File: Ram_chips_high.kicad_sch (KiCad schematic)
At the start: 10 parts, among them U25 MM5280, U26 MM5280, U27 MM5280, U28 MM5280, U40 MM5280, U41 MM5280, U42 MM5280, U43 MM5280, U6 74LS04, U7 74LS173

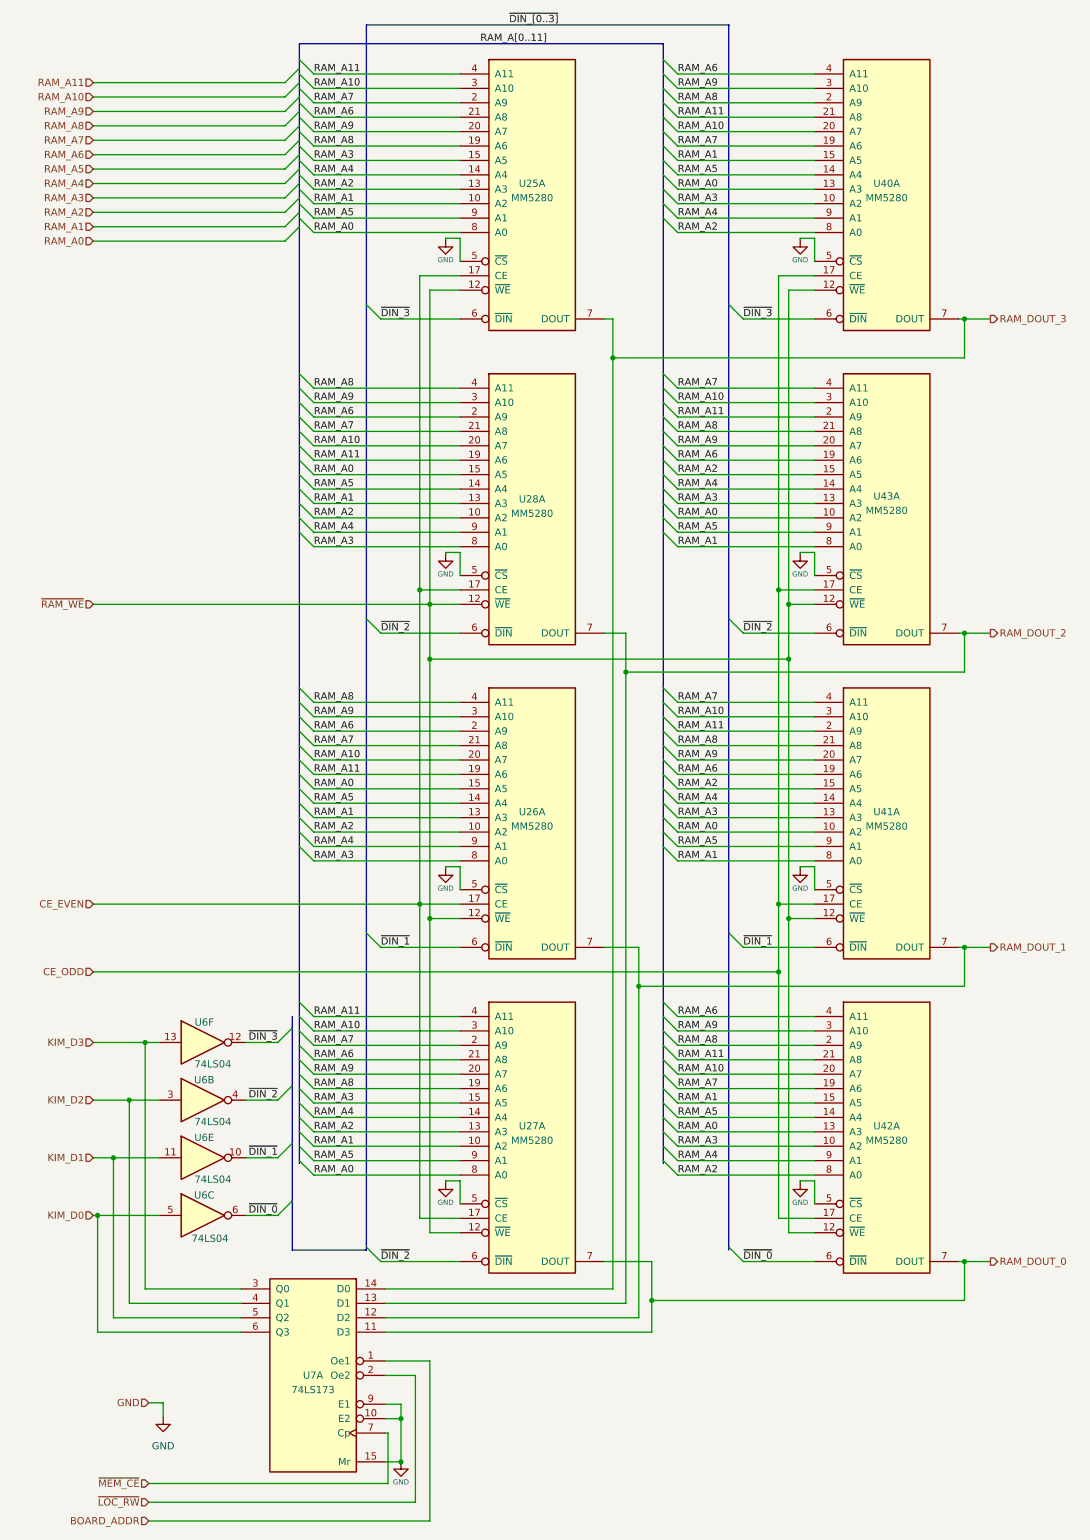
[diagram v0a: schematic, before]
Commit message: Routing completed
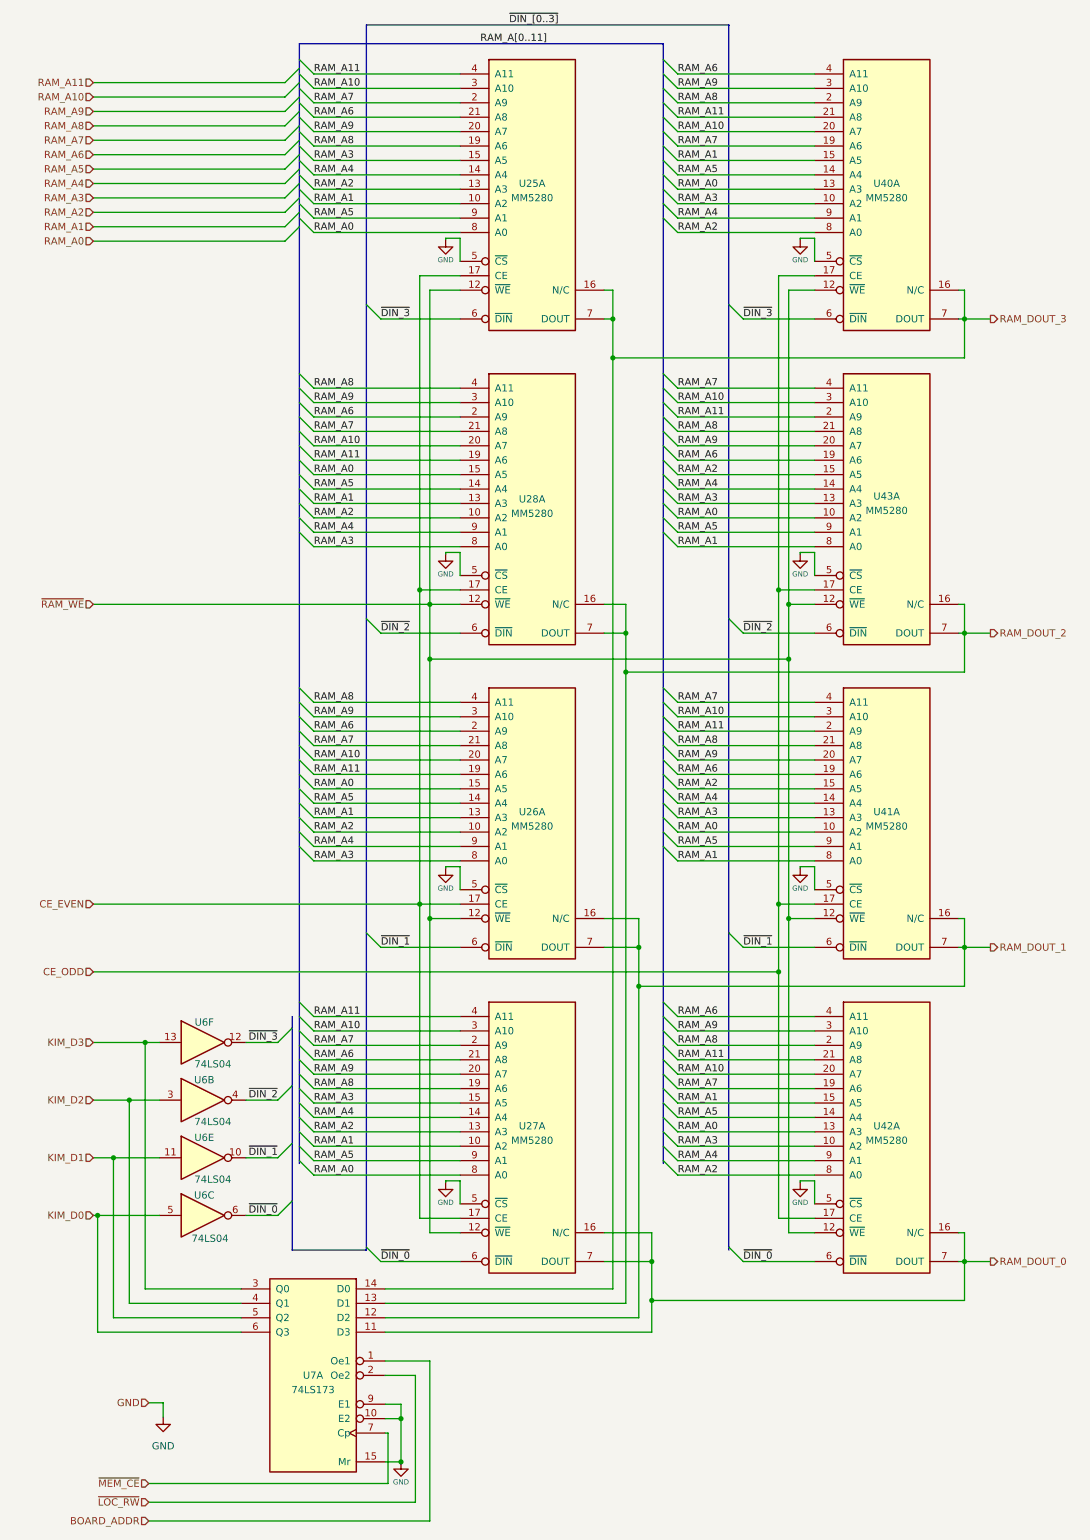
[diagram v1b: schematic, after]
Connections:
- net RAM_DOUT_0: now also U27.16 (N/C), U42.16 (N/C)
- net RAM_DOUT_1: now also U26.16 (N/C), U41.16 (N/C)
- net RAM_DOUT_2: now also U28.16 (N/C), U43.16 (N/C)
- net RAM_DOUT_3: now also U25.16 (N/C), U40.16 (N/C)
- net ~{DIN_0}: now also U27.6 (~{DIN})
- net ~{DIN_2}: no longer U27.6 (~{DIN})
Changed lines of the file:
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@@
   (junction (at 177.546 122.936) (diameter 0) (color 0 0 0 0)
   )
+  (junction (at 122.428 233.68) (diameter 0) (color 0 0 0 0)
+  )
   (junction (at 177.546 67.564) (diameter 0) (color 0 0 0 0)
   )
@@
   (junction (at 83.312 117.856) (diameter 0) (color 0 0 0 0)
   )
+  (junction (at 120.142 178.308) (diameter 0) (color 0 0 0 0)
+  )
   (junction (at 117.856 129.794) (diameter 0) (color 0 0 0 0)
   )
+  (junction (at 117.856 122.936) (diameter 0) (color 0 0 0 0)
+  )
+  (junction (at 115.57 67.564) (diameter 0) (color 0 0 0 0)
+  )
   (junction (at 144.78 170.688) (diameter 0) (color 0 0 0 0)
   )
@@
     (stroke (width 0) (type default))
   )
+  (wire (pts (xy 122.428 228.6) (xy 122.428 233.68))
+    (stroke (width 0) (type default))
+  )
   (wire (pts (xy 83.312 173.228) (xy 88.646 173.228))
     (stroke (width 0) (type default))
@@
     (stroke (width 0) (type default))
   )
+  (wire (pts (xy 176.53 117.856) (xy 177.546 117.856))
+    (stroke (width 0) (type default))
+  )
   (wire (pts (xy 148.59 164.338) (xy 148.59 164.084))
     (stroke (width 0) (type default))
@@
     (stroke (width 0) (type default))
   )
+  (wire (pts (xy 114.046 117.856) (xy 117.856 117.856))
+    (stroke (width 0) (type default))
+  )
   (wire (pts (xy 127 97.536) (xy 151.13 97.536))
     (stroke (width 0) (type default))
@@
     (stroke (width 0) (type default))
   )
+  (wire (pts (xy 176.53 228.6) (xy 177.546 228.6))
+    (stroke (width 0) (type default))
+  )
   (bus (pts (xy 72.136 65.024) (xy 72.136 120.396))
     (stroke (width 0) (type default))
@@
     (stroke (width 0) (type default))
   )
+  (wire (pts (xy 177.546 62.484) (xy 177.546 67.564))
+    (stroke (width 0) (type default))
+  )
   (wire (pts (xy 74.676 67.564) (xy 88.646 67.564))
     (stroke (width 0) (type default))
@@
     (stroke (width 0) (type default))
   )
+  (wire (pts (xy 115.57 62.484) (xy 115.57 67.564))
+    (stroke (width 0) (type default))
+  )
   (bus (pts (xy 124.46 215.9) (xy 124.46 216.408))
     (stroke (width 0) (type default))
@@
     (stroke (width 0) (type default))
   )
+  (wire (pts (xy 120.142 173.228) (xy 120.142 178.308))
+    (stroke (width 0) (type default))
+  )
   (bus (pts (xy 60.325 44.704) (xy 60.325 46.228))
     (stroke (width 0) (type default))
@@
     (stroke (width 0) (type default))
   )
+  (wire (pts (xy 177.546 173.228) (xy 177.546 178.308))
+    (stroke (width 0) (type default))
+  )
   (wire (pts (xy 62.865 140.208) (xy 88.646 140.208))
     (stroke (width 0) (type default))
@@
     (stroke (width 0) (type default))
   )
+  (wire (pts (xy 114.046 228.6) (xy 122.428 228.6))
+    (stroke (width 0) (type default))
+  )
   (bus (pts (xy 124.46 29.464) (xy 124.46 26.924))
     (stroke (width 0) (type default))
@@
     (stroke (width 0) (type default))
   )
+  (wire (pts (xy 117.856 117.856) (xy 117.856 122.936))
+    (stroke (width 0) (type default))
+  )
   (wire (pts (xy 127 107.696) (xy 151.13 107.696))
     (stroke (width 0) (type default))
@@
     (stroke (width 0) (type default))
   )
+  (wire (pts (xy 114.046 62.484) (xy 115.57 62.484))
+    (stroke (width 0) (type default))
+  )
   (wire (pts (xy 62.865 102.616) (xy 88.646 102.616))
     (stroke (width 0) (type default))
@@
     (stroke (width 0) (type default))
   )
+  (wire (pts (xy 176.53 173.228) (xy 177.546 173.228))
+    (stroke (width 0) (type default))
+  )
   (bus (pts (xy 60.325 200.66) (xy 60.325 203.2))
     (stroke (width 0) (type default))
@@
     (stroke (width 0) (type default))
   )
+  (wire (pts (xy 177.546 117.856) (xy 177.546 122.936))
+    (stroke (width 0) (type default))
+  )
+  (wire (pts (xy 177.546 228.6) (xy 177.546 233.68))
+    (stroke (width 0) (type default))
+  )
   (bus (pts (xy 60.325 105.156) (xy 60.325 132.588))
     (stroke (width 0) (type default))
@@
     (stroke (width 0) (type default))
   )
+  (wire (pts (xy 114.046 173.228) (xy 120.142 173.228))
+    (stroke (width 0) (type default))
+  )
   (wire (pts (xy 33.782 272.796) (xy 75.946 272.796))
     (stroke (width 0) (type default))
@@
   )
   (bus (pts (xy 124.46 152.908) (xy 124.46 155.448))
+    (stroke (width 0) (type default))
+  )
+  (wire (pts (xy 176.53 62.484) (xy 177.546 62.484))
     (stroke (width 0) (type default))
   )
@@
     (effects (font (size 1.27 1.27)) (justify left bottom))
   )
-  (label "~{DIN_2}" (at 74.676 233.68 0) (fields_autoplaced)
-    (effects (font (size 1.27 1.27)) (justify left bottom))
-  )
+  (label "~{DIN_0}" (at 74.676 233.68 0) (fields_autoplaced)
+    (effects (font (size 1.27 1.27)) (justify left bottom))
+  )
